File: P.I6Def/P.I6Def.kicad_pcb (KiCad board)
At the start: 2 copper layers, 48.9 x 70.8 mm, 41 parts, among them J1 B3B-PH-K-S, J2 B3B-PH-K-S, J3 CX90B-16P1, J4 B4B-PH-SM4-TB_LF__SN__P_, J5 B4B-PH-SM4-TB_LF__SN__P_, SW2 SW_SPST, SW3 SW_SPST, U2 LMV321IDCKT, U3 LMV321IDCKT, U4 LMV321IDCKT, U5 LMV321IDCKT, X1 ESP32-S3-WROOM-1-N16R8

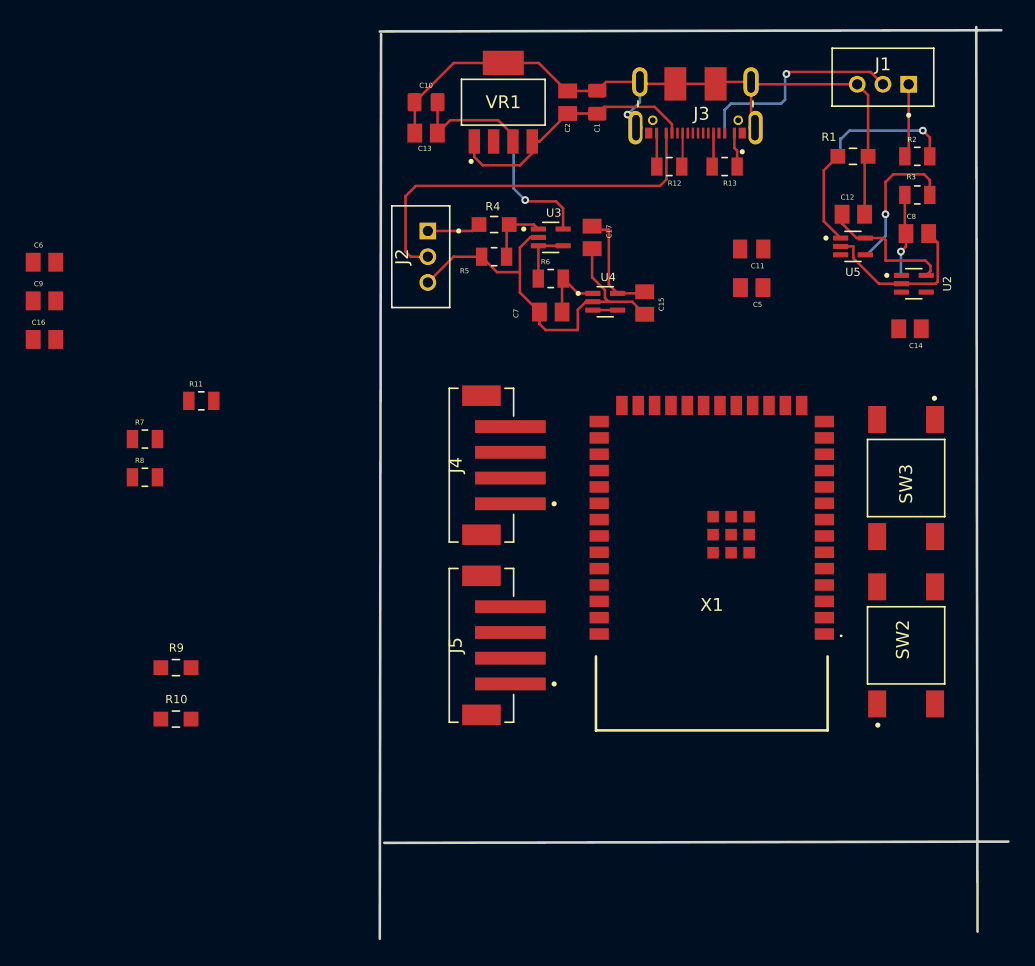
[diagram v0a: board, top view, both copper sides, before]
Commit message: MEJORA DE LA PCB
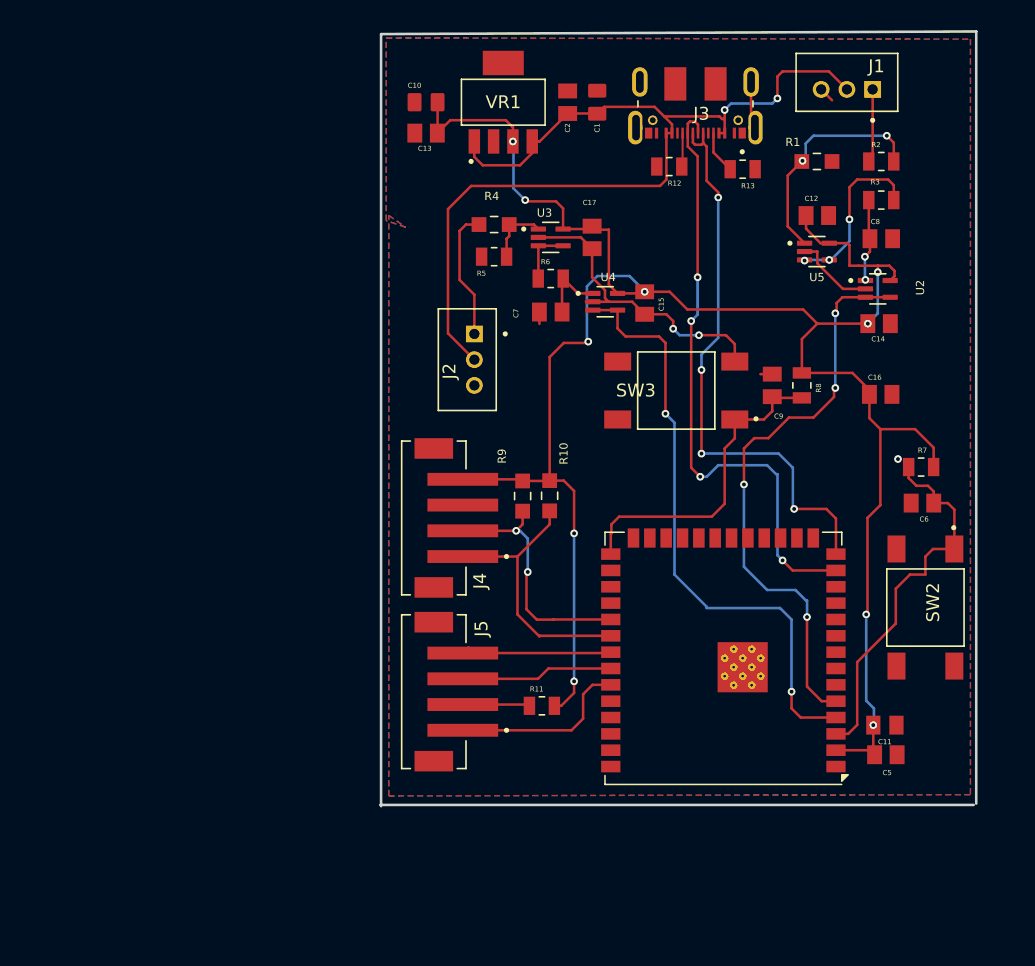
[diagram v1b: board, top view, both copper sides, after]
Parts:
- removed X1: ESP32-S3-WROOM-1-N16R8, ESP32-S3-WROOM-1-N16R8:ESP32S3WROOM1N8R2
- added U6: ESP32-S3-WROOM-1, RF_Module:ESP32-S3-WROOM-1U, F.Cu at (126.8, 93.2)
- moved C6 70.7 mm to (142.3, 81.1), turned to 180 degrees
- moved C16 65.1 mm to (139.0, 72.7)
- moved R7 60.4 mm to (142.2, 78.3), turned to 180 degrees
- moved C9 56.9 mm to (130.6, 72.0), turned to 90 degrees
- moved R8 51.5 mm to (132.9, 72.0), turned to 90 degrees
- moved C11 38.4 mm to (139.3, 98.4), turned to 0 degrees
- moved C5 37.8 mm to (139.4, 100.7), turned to 0 degrees
- moved R11 35.5 mm to (112.7, 96.9)
- moved R10 33.8 mm to (113.3, 80.6), turned to -90 degrees
- moved R9 30.1 mm to (111.2, 80.6), turned to -90 degrees
- moved SW3 19.1 mm to (123.1, 72.4), turned to 180 degrees
- moved J2 8.78 mm to (106.9, 70.0)
- moved J4 5.52 mm to (104.3, 82.3)
- moved J5 5.16 mm to (104.3, 95.8)
- moved SW2 3.30 mm to (142.5, 89.3), turned to -90 degrees
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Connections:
- net Net-(SW3-A) renamed /BOOT
- C1 pad 1: VBUS_B -> +5V
- C2 pad 1: VBUS_B -> +5V
- J3 pad B4: VBUS_B -> +5V
- J3 pad B9: VBUS_B -> +5V
- VR1 pad 1: VBUS_B -> +5V
- VR1 pad 4: VBUS_B -> +5V
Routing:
- net +3.3V: track 39.2 -> 164.0 mm, vias 1 -> 10
- net GND: track 109.2 -> 42.5 mm, vias 1 -> 3
- net /D-: track 0.00 -> 47.9 mm, vias 0 -> 4
- net /ADC1_CH1: track 1.92 -> 47.1 mm, vias 0 -> 2
- net /ADC1_CH0: track 0.00 -> 45.0 mm, vias 0 -> 4
- net /D+: track 0.00 -> 44.7 mm, vias 0 -> 4
- net Net-(SW2-A): track 0.00 -> 29.4 mm
- net +5V: track 47.4 -> 74.4 mm, vias 1 -> 2
- net /BOOT: track 0.00 -> 25.3 mm
- net /SCL_CSS811: track 0.00 -> 21.3 mm
- net VBUS_B: track 20.5 -> 0.00 mm
- net /SDA_CSS811: track 0.00 -> 19.5 mm, vias 0 -> 2
- net /ADDR_CCS811: track 0.00 -> 14.1 mm
- net /WAKE_CCS811: track 0.00 -> 12.2 mm
- net /nINT_CCS811: track 0.00 -> 11.8 mm
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- added copper zone on B.Cu, net GND
- added copper zone on F.Cu, net GND
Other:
- board size 48.9 x 70.8 mm -> 46.3 x 60.2 mm
